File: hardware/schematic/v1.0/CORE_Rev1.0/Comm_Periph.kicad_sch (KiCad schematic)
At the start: 20 parts, among them J1 Conn_01x06_Socket, J11 Conn_01x06_Socket, J13 Conn_01x04_Socket, J14 Conn_01x03_Socket, J15 Conn_01x05_Socket, J16 Conn_01x04_Socket

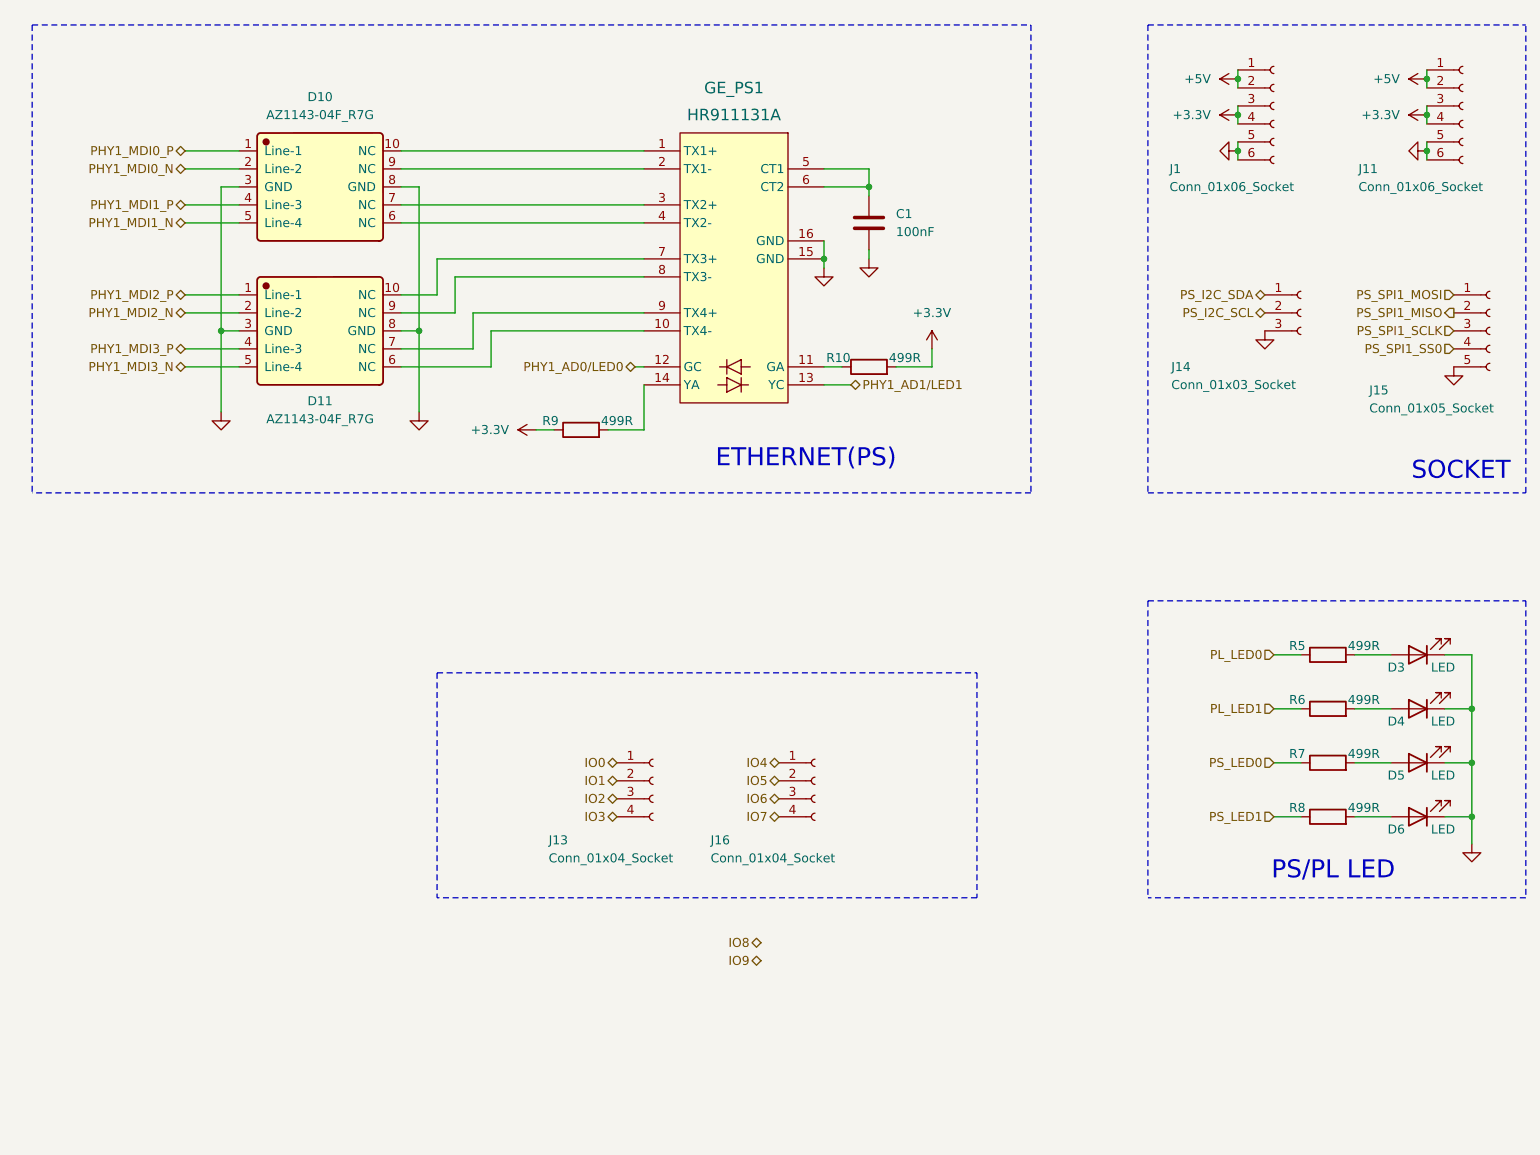
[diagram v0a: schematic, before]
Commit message: sch update
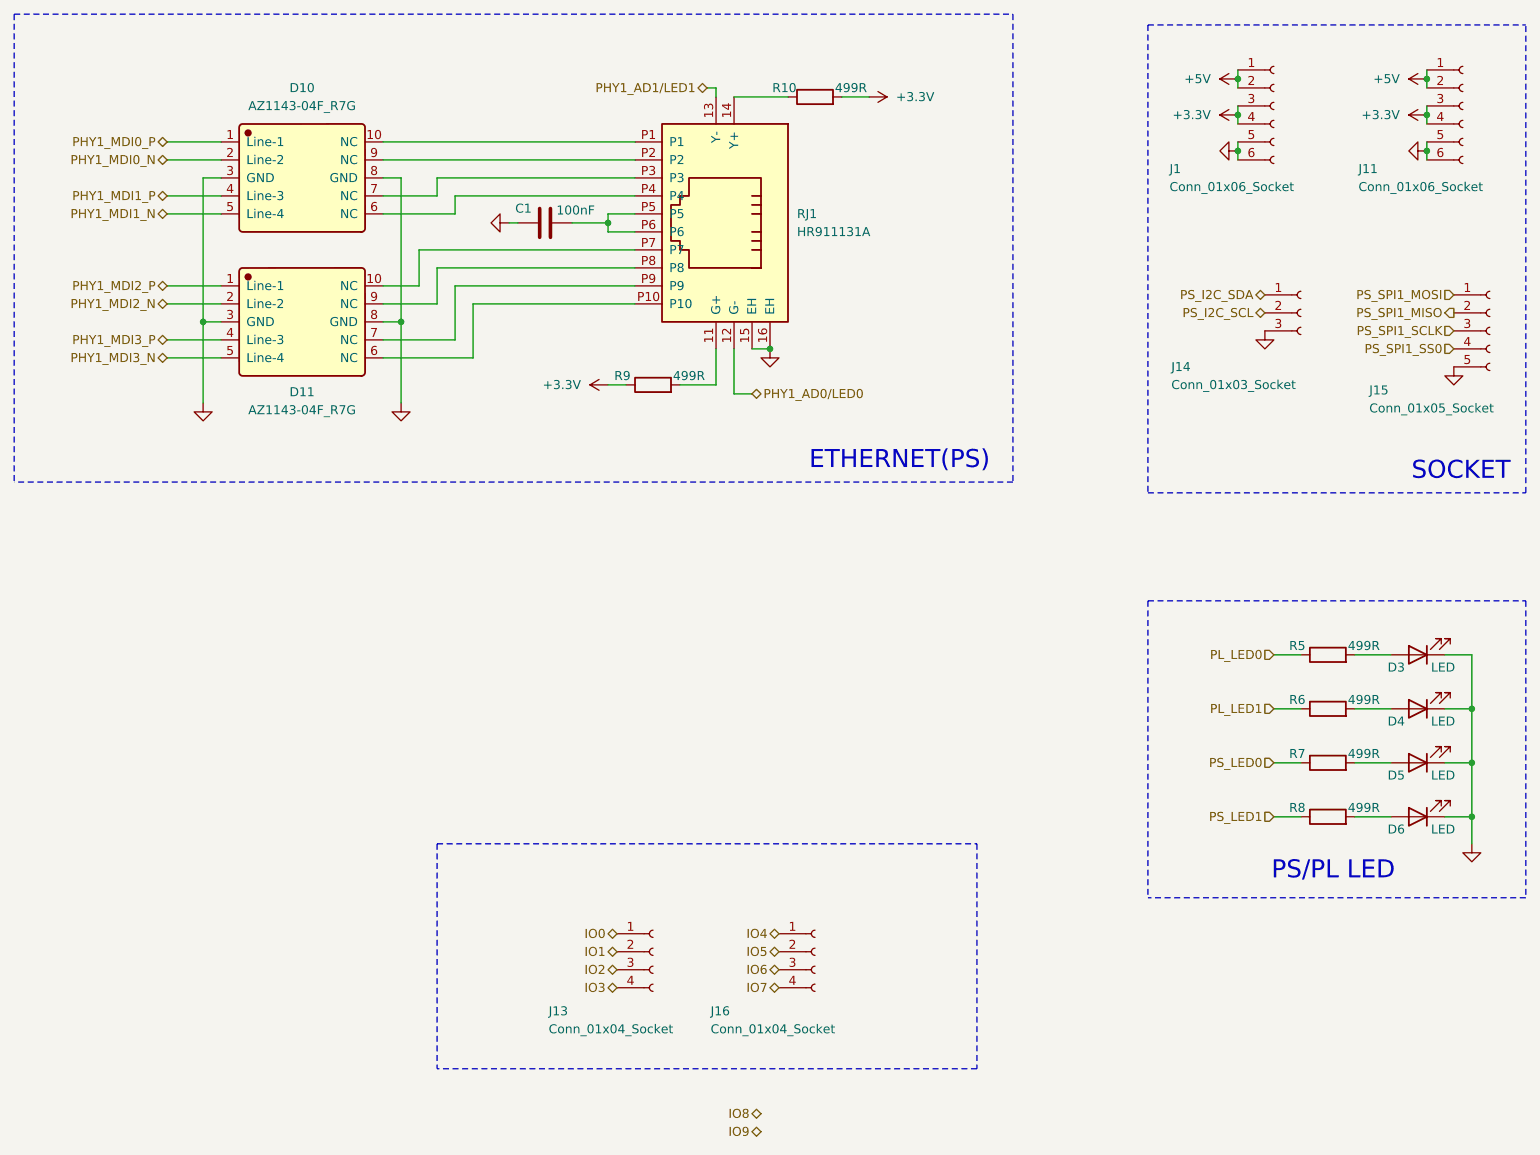
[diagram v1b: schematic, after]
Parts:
- removed GE_PS1: HR911131A, Counter:HR911131A, symbol Counter:HR911131A_C
- added RJ1: HR911131A, CORE:HR911131A, symbol CORE:HR911131A
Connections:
- net GND: now also C1.1, RJ1.15 (EH), RJ1.16 (EH); no longer C1.2
- net PHY1_AD0/LED0: now also RJ1.12 (G-)
- net PHY1_AD1/LED1: now also RJ1.13 (Y-)
- net at R10.1: now also RJ1.14 (Y+)
- net at D11.10 (NC): now also RJ1.P7
- net at D11.6 (NC): now also RJ1.P10
- net at D11.7 (NC): now also RJ1.P9
- net at D11.9 (NC): now also RJ1.P8
- net at R9.2: now also RJ1.11 (G+)
- net at D10.10 (NC): now also RJ1.P1
- net at D10.9 (NC): now also RJ1.P2
- net at D10.7 (NC): now also RJ1.P3
- net at D10.6 (NC): now also RJ1.P4
- new net: C1.2, RJ1.P5, RJ1.P6
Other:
- moved on the sheet: D10, D11, J13, J16, R10, R9

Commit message: sch update
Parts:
- C1: footprint Capacitor_SMD:C_0402_1005Metric -> CORE:C_0402_1005Metric; symbol Device:C -> CORE:C
- D3, D4, D5, D6: footprint LED_SMD:LED_0603_1608Metric -> CORE:LED_0603_1608Metric; symbol Device:LED -> CORE:LED
- R10, R5, R6, R7, R8, R9: footprint Resistor_SMD:R_0402_1005Metric -> CORE:R_0402_1005Metric; symbol Device:R -> CORE:R
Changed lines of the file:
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@@
 	)
 	(symbol
-		(lib_id "Device:R")
+		(lib_id "CORE:R")
 		(at 140.97 41.91 90)
 		(unit 1)
@@
 			)
 		)
-		(property "Footprint" "Resistor_SMD:R_0402_1005Metric"
+		(property "Footprint" "CORE:R_0402_1005Metric"
 			(at 140.97 43.688 90)
 			(hide yes)
@@
 	)
 	(symbol
-		(lib_id "Device:LED")
+		(lib_id "CORE:LED")
 		(at 226.06 128.27 180)
 		(unit 1)
@@
 			)
 		)
-		(property "Footprint" "LED_SMD:LED_0603_1608Metric"
+		(property "Footprint" "CORE:LED_0603_1608Metric"
 			(at 226.06 128.27 0)
 			(hide yes)
@@
 	)
 	(symbol
-		(lib_id "Device:C")
+		(lib_id "CORE:C")
 		(at 102.87 59.69 90)
 		(unit 1)
@@
 			)
 		)
-		(property "Footprint" "Capacitor_SMD:C_0402_1005Metric"
+		(property "Footprint" "CORE:C_0402_1005Metric"
 			(at 106.68 58.7248 0)
 			(hide yes)
@@
 	)
 	(symbol
-		(lib_id "Device:LED")
+		(lib_id "CORE:LED")
 		(at 226.06 143.51 180)
 		(unit 1)
@@
 			)
 		)
-		(property "Footprint" "LED_SMD:LED_0603_1608Metric"
+		(property "Footprint" "CORE:LED_0603_1608Metric"
 			(at 226.06 143.51 0)
 			(hide yes)
@@
 	)
 	(symbol
-		(lib_id "Device:LED")
+		(lib_id "CORE:LED")
 		(at 226.06 135.89 180)
 		(unit 1)
@@
 			)
 		)
-		(property "Footprint" "LED_SMD:LED_0603_1608Metric"
+		(property "Footprint" "CORE:LED_0603_1608Metric"
 			(at 226.06 135.89 0)
 			(hide yes)
@@
 	)
 	(symbol
-		(lib_id "Device:R")
+		(lib_id "CORE:R")
 		(at 213.36 143.51 90)
 		(unit 1)
@@
 			)
 		)
-		(property "Footprint" "Resistor_SMD:R_0402_1005Metric"
+		(property "Footprint" "CORE:R_0402_1005Metric"
 			(at 213.36 145.288 90)
 			(hide yes)
@@
 	)
 	(symbol
-		(lib_id "Device:R")
+		(lib_id "CORE:R")
 		(at 213.36 120.65 90)
 		(unit 1)
@@
 			)
 		)
-		(property "Footprint" "Resistor_SMD:R_0402_1005Metric"
+		(property "Footprint" "CORE:R_0402_1005Metric"
 			(at 213.36 122.428 90)
 			(hide yes)
@@
 	)
 	(symbol
-		(lib_id "Device:R")
+		(lib_id "CORE:R")
 		(at 213.36 135.89 90)
 		(unit 1)
@@
 			)
 		)
-		(property "Footprint" "Resistor_SMD:R_0402_1005Metric"
+		(property "Footprint" "CORE:R_0402_1005Metric"
 			(at 213.36 137.668 90)
 			(hide yes)
@@
 	)
 	(symbol
-		(lib_id "Device:LED")
+		(lib_id "CORE:LED")
 		(at 226.06 120.65 180)
 		(unit 1)
@@
 			)
 		)
-		(property "Footprint" "LED_SMD:LED_0603_1608Metric"
+		(property "Footprint" "CORE:LED_0603_1608Metric"
 			(at 226.06 120.65 0)
 			(hide yes)
@@
 	)
 	(symbol
-		(lib_id "Device:R")
+		(lib_id "CORE:R")
 		(at 118.11 82.55 90)
 		(unit 1)
@@
 			)
 		)
-		(property "Footprint" "Resistor_SMD:R_0402_1005Metric"
+		(property "Footprint" "CORE:R_0402_1005Metric"
 			(at 118.11 84.328 90)
 			(hide yes)
@@
 	)
 	(symbol
-		(lib_id "Device:R")
+		(lib_id "CORE:R")
 		(at 213.36 128.27 90)
 		(unit 1)
@@
 			)
 		)
-		(property "Footprint" "Resistor_SMD:R_0402_1005Metric"
+		(property "Footprint" "CORE:R_0402_1005Metric"
 			(at 213.36 130.048 90)
 			(hide yes)
